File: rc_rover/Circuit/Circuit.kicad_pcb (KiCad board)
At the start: 2 copper layers, 22 parts, among them J1 Barrel_Jack_MountingPin, U1 L7805, U2 L298N, U3 LM317, U4 NRF24L01_Breakout

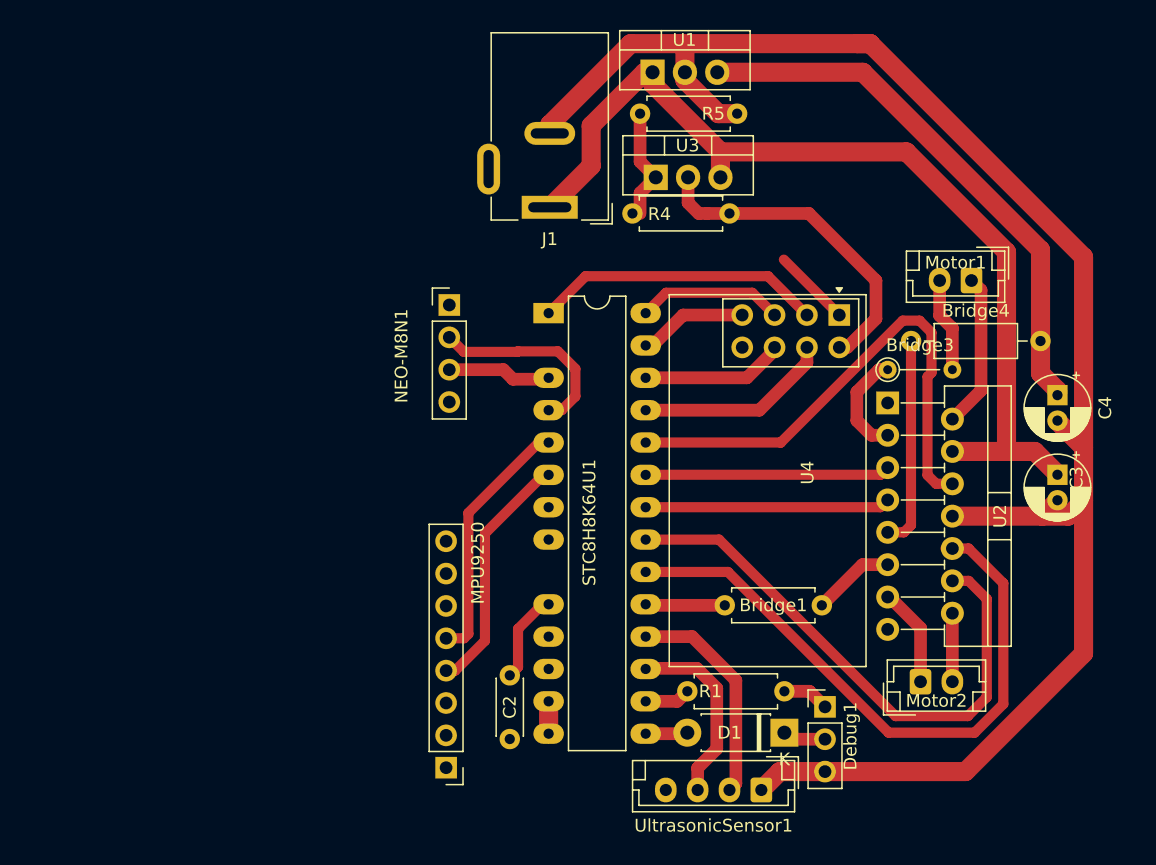
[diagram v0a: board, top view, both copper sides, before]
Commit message: finished circuit schematic and PCB layout
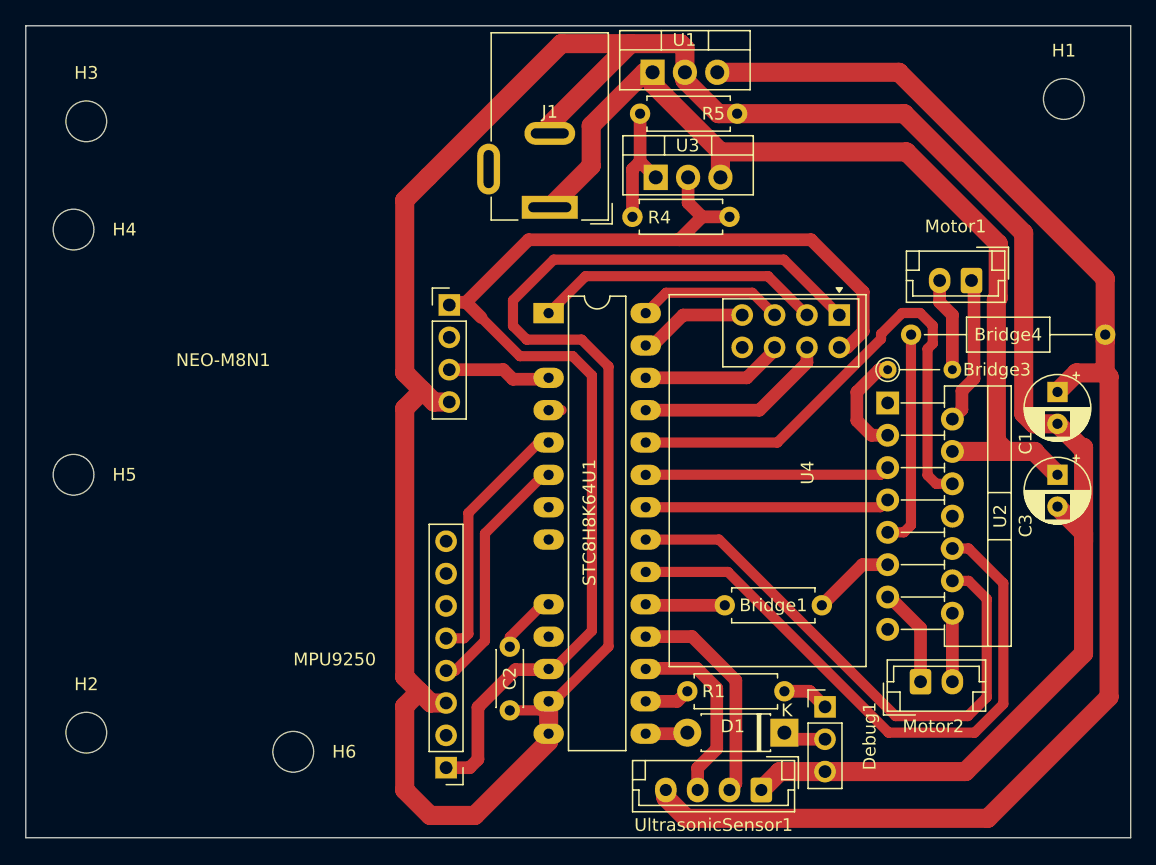
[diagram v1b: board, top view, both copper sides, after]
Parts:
- removed C4: 100nF, Capacitor_THT:CP_Radial_D5.0mm_P2.00mm
- added C1: 100nF, Capacitor_THT:CP_Radial_D5.0mm_P2.50mm, F.Cu at (156.2, 75.2)
- added H1: 3.2mm, MountingHole:MountingHole_3.2mm_M3_DIN965, F.Cu at (156.8, 52.2)
- added H2: 3.2mm, MountingHole:MountingHole_3.2mm_M3_DIN965, F.Cu at (80.0, 102.0)
- added H3: 3.2mm, MountingHole:MountingHole_3.2mm_M3_DIN965, F.Cu at (80.0, 54.0)
- added H4: 3.2mm, MountingHole:MountingHole_3.2mm_M3_DIN965, F.Cu at (79.0, 62.5)
- added H5: 3.2mm, MountingHole:MountingHole_3.2mm_M3_DIN965, F.Cu at (79.0, 81.8)
- added H6: 3.2mm, MountingHole:MountingHole_3.2mm_M3_DIN965, F.Cu at (96.2, 103.5)
- Bridge4: footprint Resistor_THT:R_Axial_DIN0207_L6.3mm_D2.5mm_P10.16mm_Horizontal -> Resistor_THT:R_Axial_DIN0207_L6.3mm_D2.5mm_P15.24mm_Horizontal
- C3: footprint Capacitor_THT:CP_Radial_D5.0mm_P2.00mm -> Capacitor_THT:CP_Radial_D5.0mm_P2.50mm
- J1: value Barrel_Jack_MountingPin -> Barrel_Jack
- moved C2 2.25 mm to (113.2, 95.2)
- moved Bridge4 0.50 mm to (144.8, 70.8)
- moved R4 0.27 mm to (122.9, 61.5)
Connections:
- NEO-M8N1 pad 2: RX -> unconnected-(NEO-M8N1-Pin_2-Pad2)
- STC8H8K64U1 pad 4: RX -> unconnected-(STC8H8K64U1-Pin_4-Pad4)
- UltrasonicSensor1 pad 4: +3.3V -> +5V
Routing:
- net GND: track 147.1 -> 283.6 mm
- net +3.3V: track 26.9 -> 100.8 mm
- net +5V: track 43.1 -> 114.7 mm
- net RX: track 16.1 -> 0.00 mm
- net Net-(STC8H8K64U1-Pin_10): track 7.52 -> 5.27 mm
- net unconnected-(STC8H8K64U1-Pin_4-Pad4): track 0.00 -> 1.43 mm
- net Net-(U3-ADJ): track 8.85 -> 10.1 mm
- net EnA: track 40.3 -> 41.5 mm
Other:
- board outline added: 86.8 x 63.8 mm
